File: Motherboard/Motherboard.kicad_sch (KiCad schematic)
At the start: 6 parts

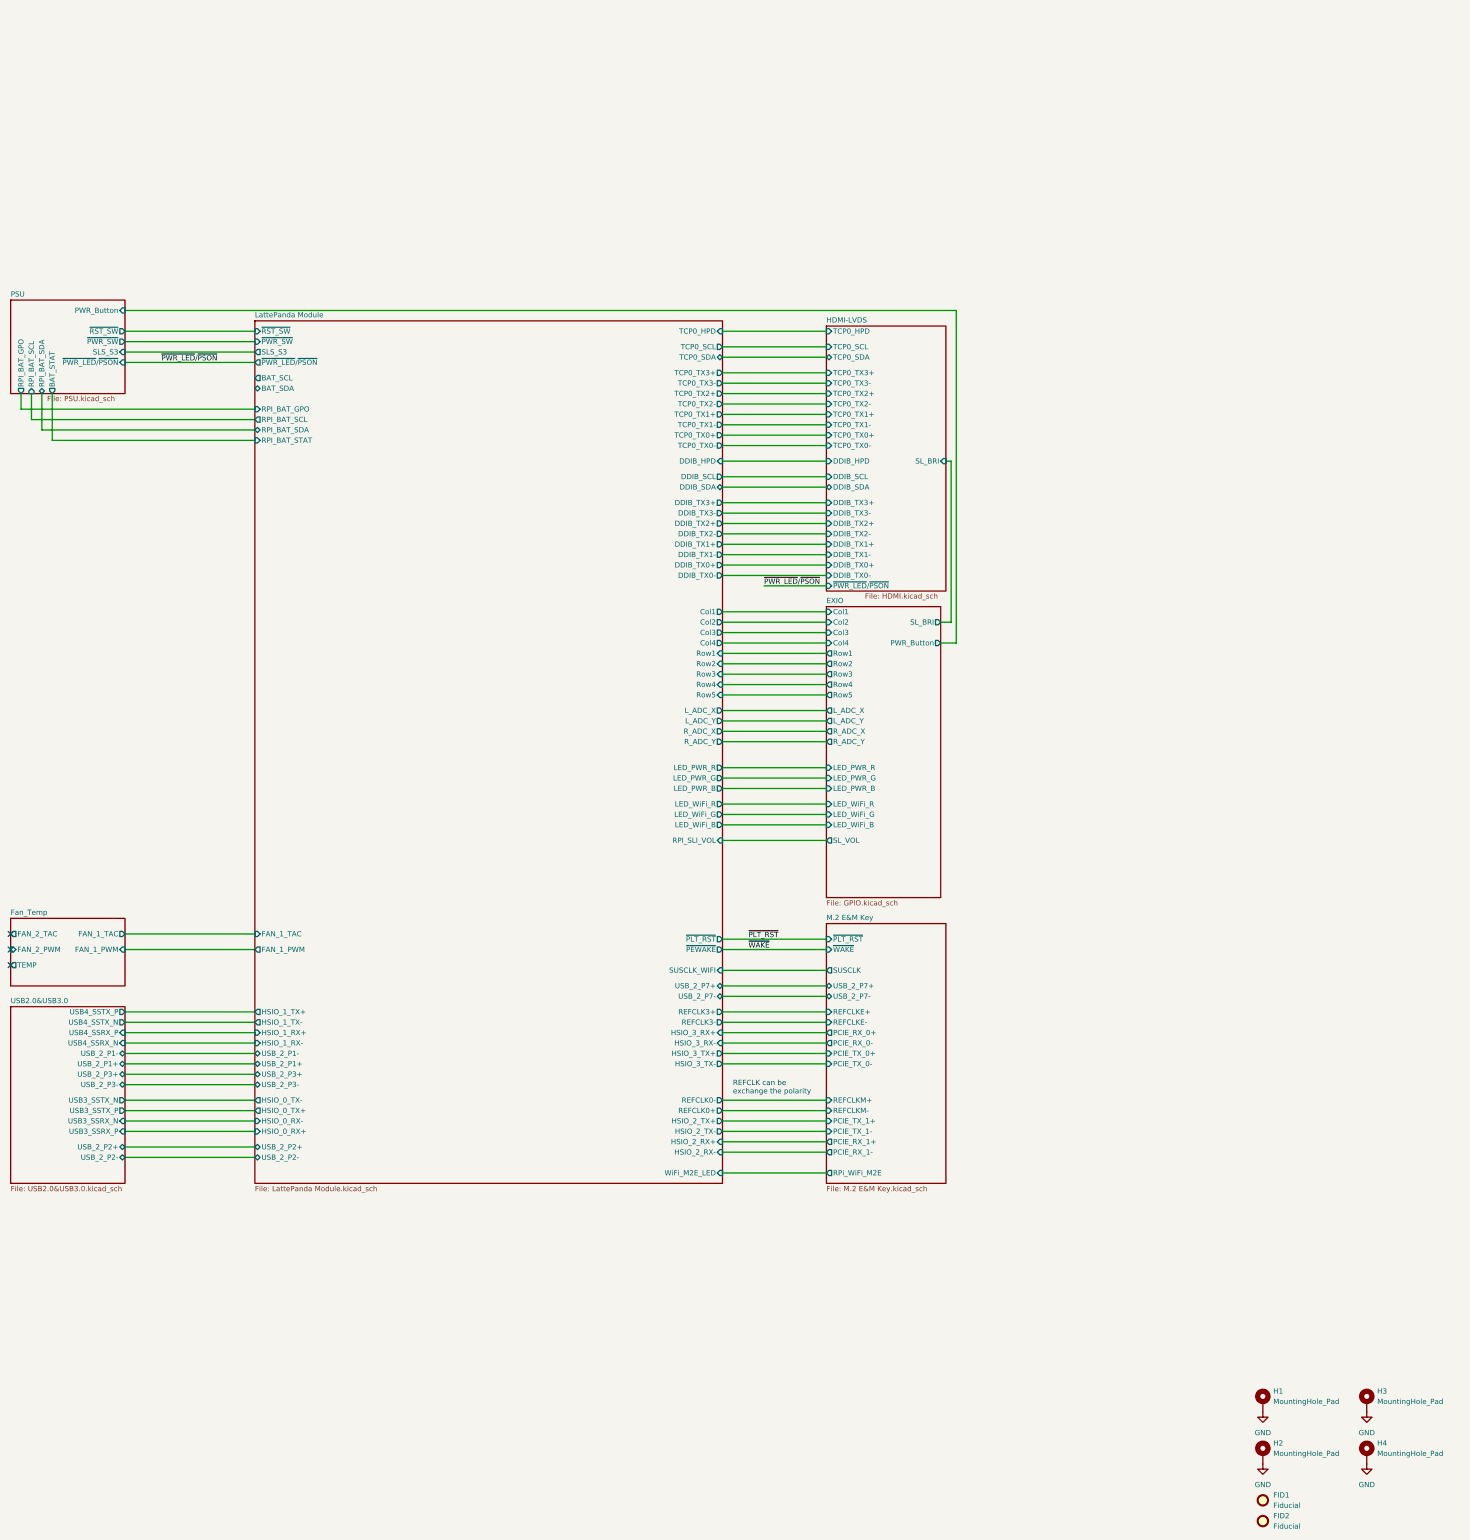
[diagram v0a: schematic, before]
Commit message: Switched HDMI DBUG and TCP0 back, added I2C Protection circuits, and a lot more random changes/updates/progress
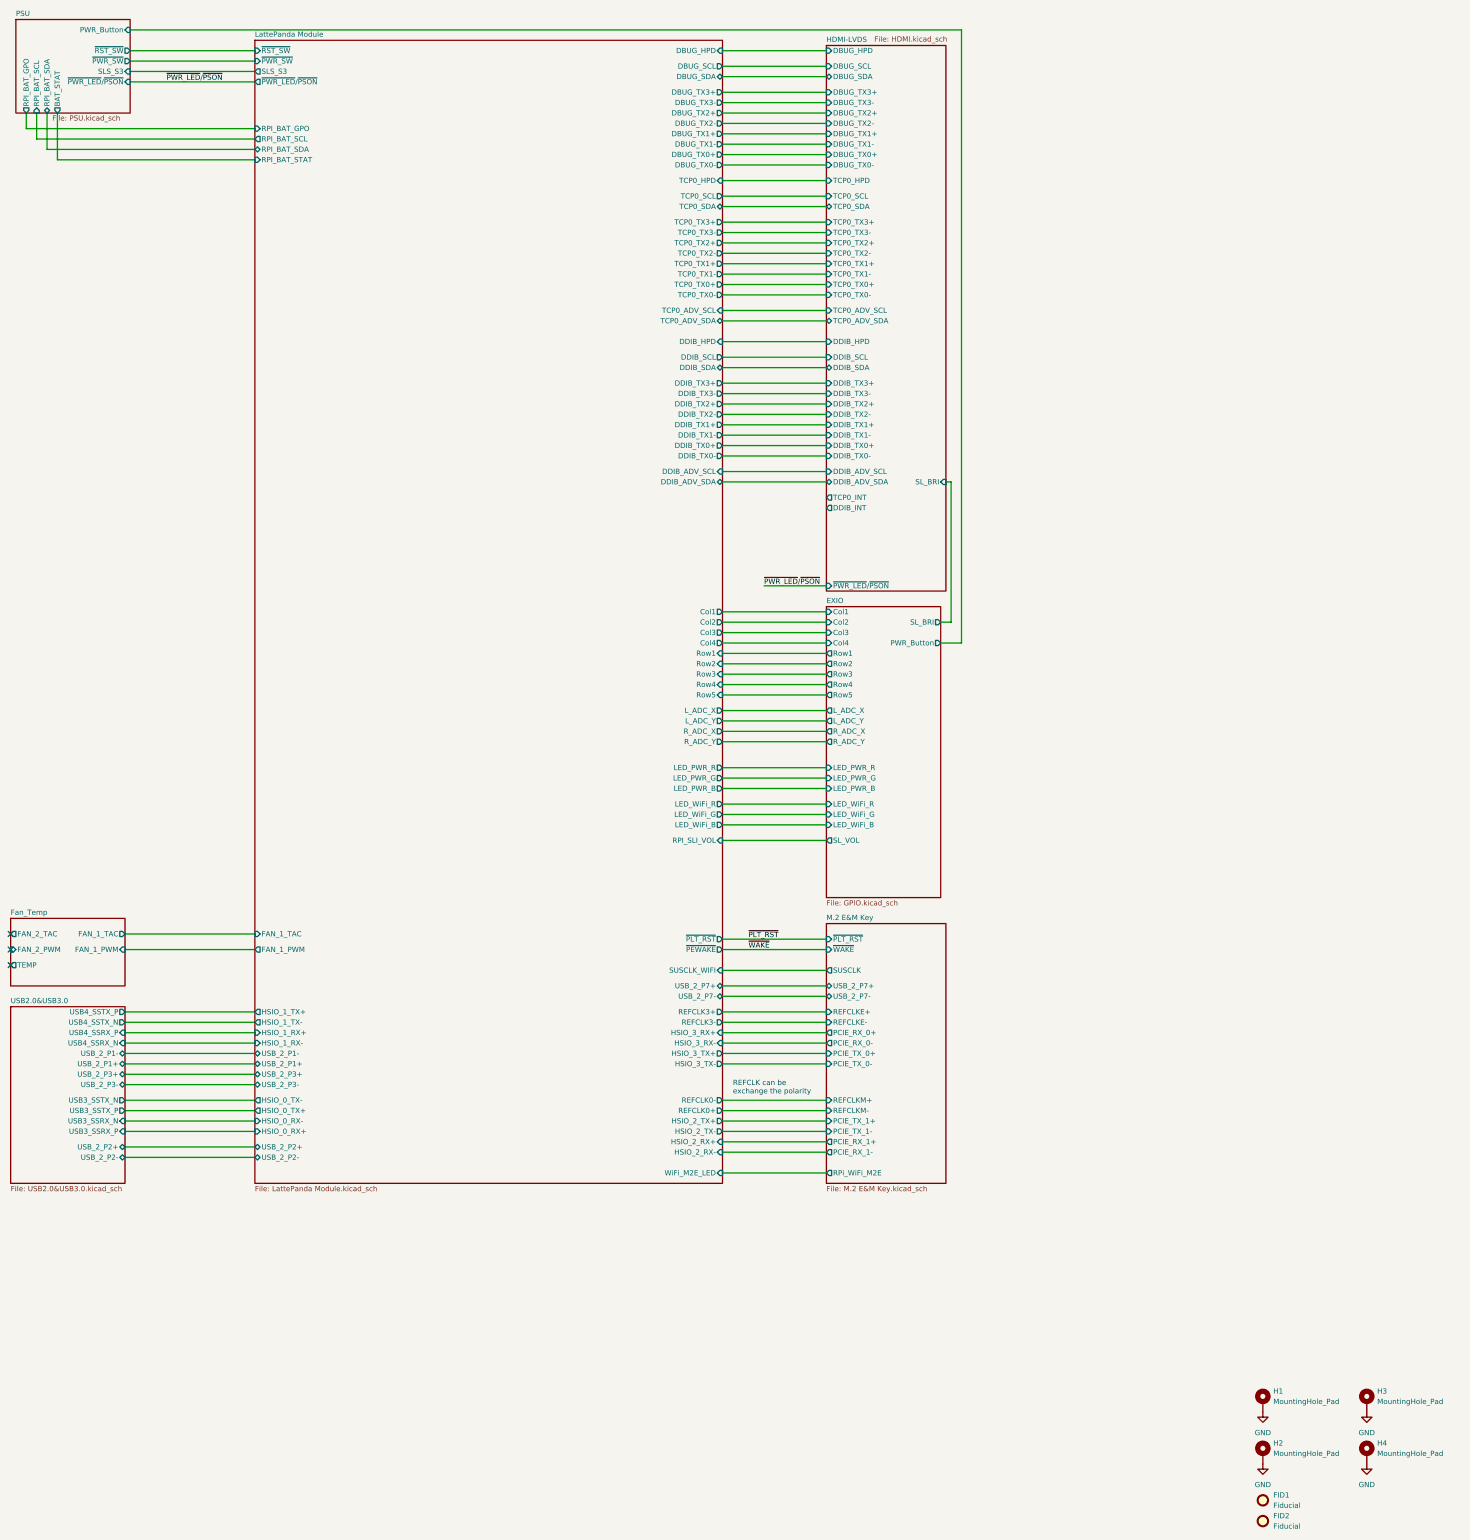
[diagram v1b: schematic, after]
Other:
- sheet HDMI-LVDS ports: added DBUG_HPD, DBUG_SCL, DBUG_SDA, DBUG_TX0+, DBUG_TX0-, DBUG_TX1+, DBUG_TX1-, DBUG_TX2+, DBUG_TX2-, DBUG_TX3+, DBUG_TX3-, DDIB_ADV_SCL, DDIB_ADV_SDA, DDIB_INT, TCP0_ADV_SCL, TCP0_ADV_SDA, TCP0_INT; removed none
- sheet LattePanda Module ports: added DBUG_HPD, DBUG_SCL, DBUG_SDA, DBUG_TX0+, DBUG_TX0-, DBUG_TX1+, DBUG_TX1-, DBUG_TX2+, DBUG_TX2-, DBUG_TX3+, DBUG_TX3-, DDIB_ADV_SCL, DDIB_ADV_SDA, TCP0_ADV_SCL, TCP0_ADV_SDA; removed BAT_SCL, BAT_SDA
